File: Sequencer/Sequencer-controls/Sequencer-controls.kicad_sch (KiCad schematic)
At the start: 14 parts, among them SW1 SW_Push_DPDT, SW2 SW_Rotary3x4, SW3 SW_Rotary12

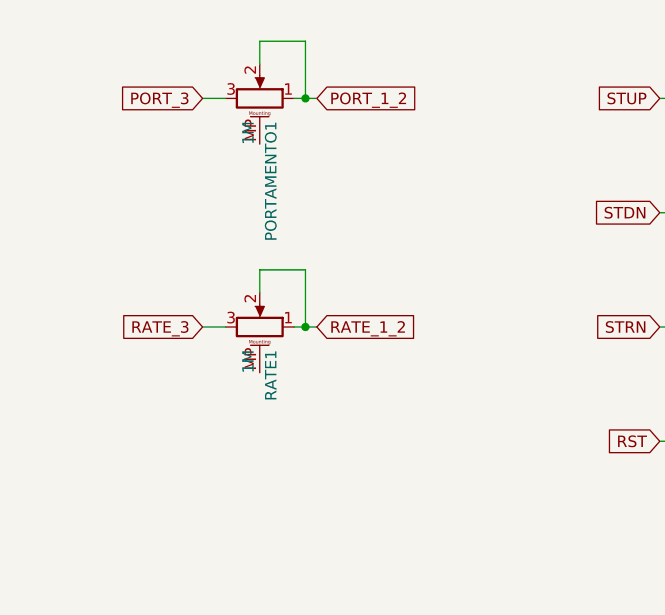
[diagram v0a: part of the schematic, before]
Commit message: Sequencer control - minor
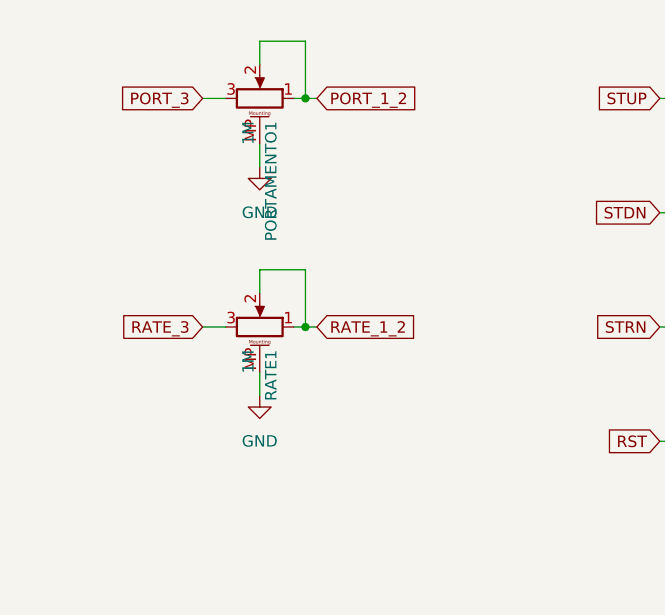
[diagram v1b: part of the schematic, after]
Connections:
- net GND: now also PORTAMENTO1.MP (MountPin), RATE1.MP (MountPin)
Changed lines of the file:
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@@
+    (stroke (width 0) (type default))
+  )
+  (wire (pts (xy 41.91 55.88) (xy 41.91 58.42))
     (stroke (width 0) (type default))
   )
@@
     (stroke (width 0) (type default))
   )
+  (wire (pts (xy 41.91 30.48) (xy 41.91 33.02))
+    (stroke (width 0) (type default))
+  )
   (wire (pts (xy 46.99 44.45) (xy 46.99 50.8))
     (stroke (width 0) (type default))
@@
         (path "/0fe7de3d-0e02-4720-a37d-4e739d042412"
           (reference "#PWR03") (unit 1)
+        )
+      )
+    )
+  )
+  (symbol (lib_id "power:GND") (at 41.91 33.02 0) (unit 1)
+    (in_bom yes) (on_board yes) (dnp no) (fields_autoplaced)
+    (property "Reference" "#PWR079" (at 41.91 39.37 0)
+      (effects (font (size 1.27 1.27)) hide)
+    )
+    (property "Value" "GND" (at 41.91 38.1 0)
+      (effects (font (size 1.27 1.27)))
+    )
+    (property "Footprint" "" (at 41.91 33.02 0)
+      (effects (font (size 1.27 1.27)) hide)
+    )
+    (property "Datasheet" "" (at 41.91 33.02 0)
+      (effects (font (size 1.27 1.27)) hide)
+    )
+    (pin "1")
+    (instances
+      (project "Sequencer-controls"
+        (path "/0fe7de3d-0e02-4720-a37d-4e739d042412"
+          (reference "#PWR079") (unit 1)
         )
       )
@@
         )
       )
+    )
+  )
+  (symbol (lib_id "power:GND") (at 41.91 58.42 0) (unit 1)
+    (in_bom yes) (on_board yes) (dnp no) (fields_autoplaced)
+    (property "Reference" "#PWR078" (at 41.91 64.77 0)
+      (effects (font (size 1.27 1.27)) hide)
+    )
+    (property "Value" "GND" (at 41.91 63.5 0)
+      (effects (font (size 1.27 1.27)))
+    )
+    (property "Footprint" "" (at 41.91 58.42 0)
+      (effects (font (size 1.27 1.27)) hide)
+    )
+    (property "Datasheet" "" (at 41.91 58.42 0)
+      (effects (font (size 1.27 1.27)) hide)
+    )
+    (pin "1")
+    (instances
+      (project "Sequencer-controls"
+        (path "/0fe7de3d-0e02-4720-a37d-4e739d042412"
+          (reference "#PWR078") (unit 1)
+        )
+      )
